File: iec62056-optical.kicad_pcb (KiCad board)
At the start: 2 copper layers, 30 x 30 mm, 5 parts, among them J1 Conn_01x04_Male, Q1 Q_Photo_NPN

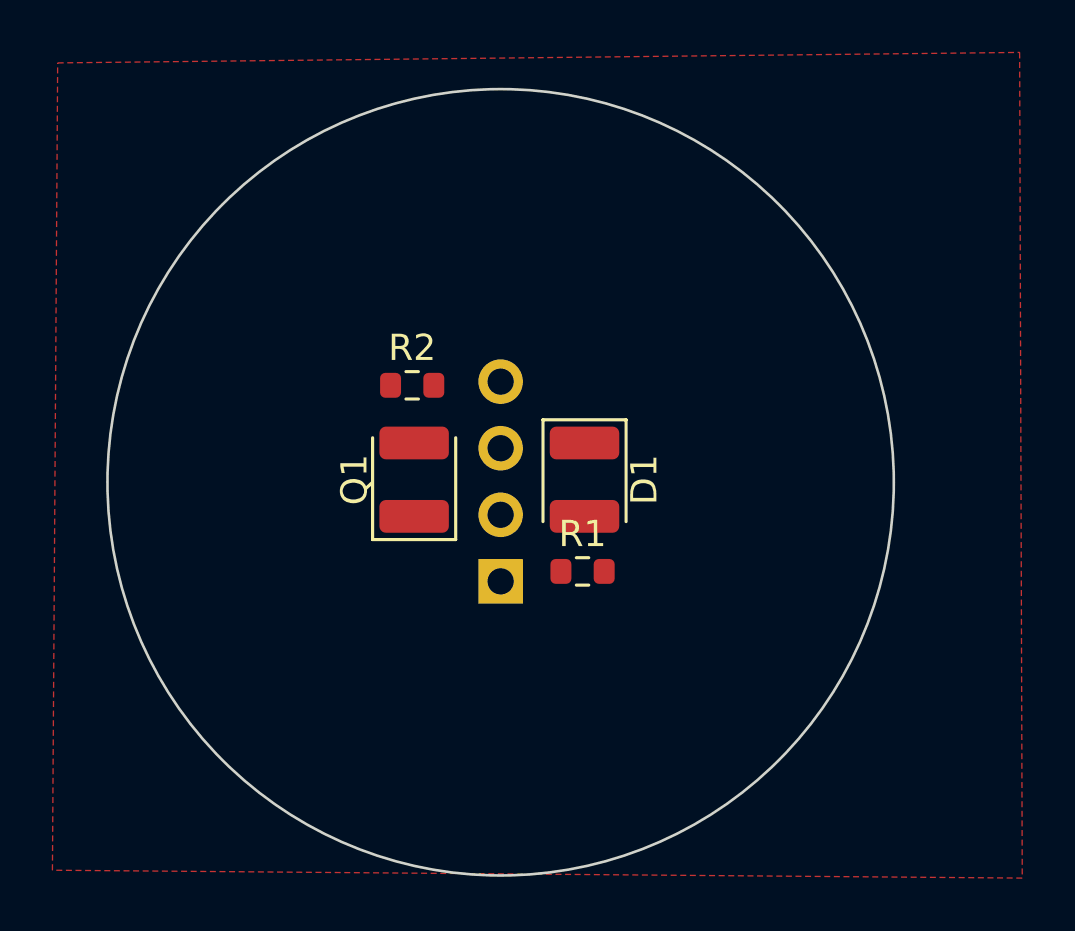
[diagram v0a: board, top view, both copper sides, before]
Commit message: version 1.0
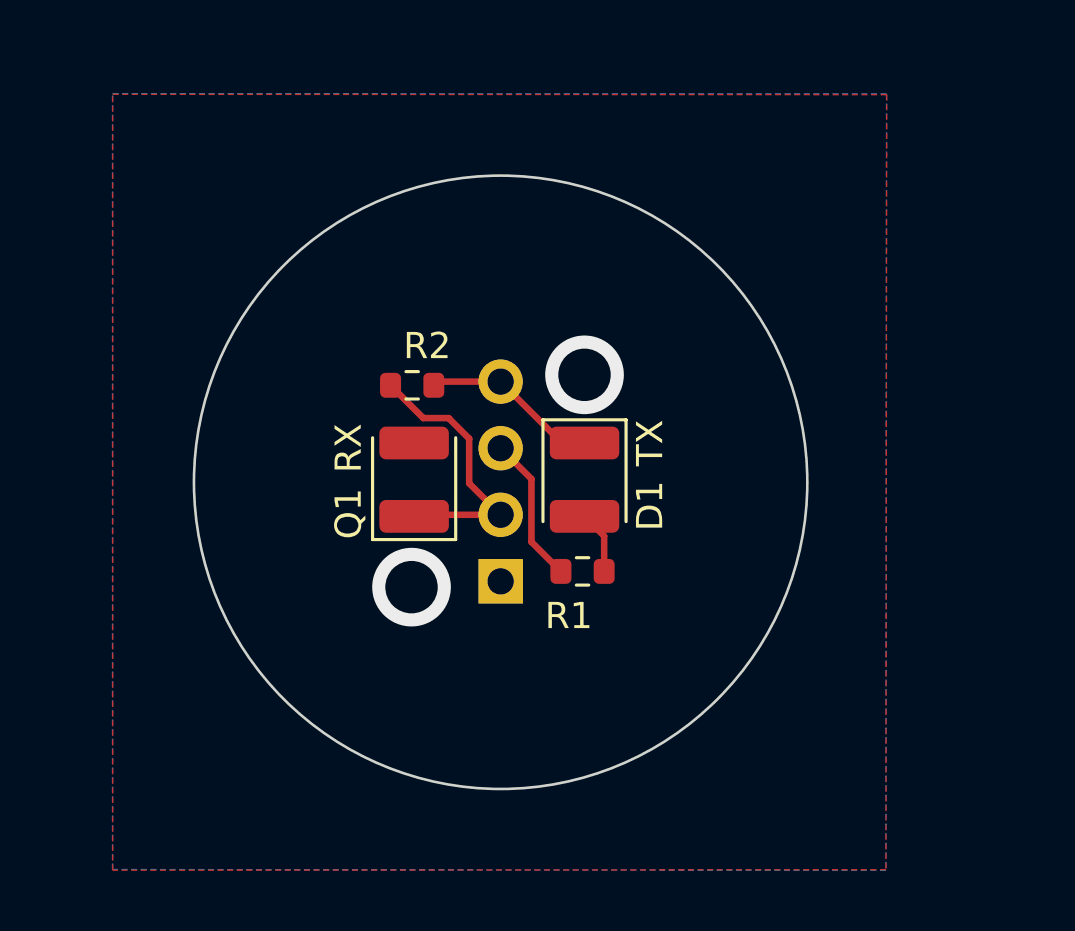
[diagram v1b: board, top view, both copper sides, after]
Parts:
- D1: value LED -> IR42-21C
- Q1: value Q_Photo_NPN -> PT42-21B
- R1: value R -> 0R
- R2: value R -> 1k8
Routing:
- net RXD: track 0.00 -> 10.6 mm
- net +3V3: track 0.00 -> 6.78 mm
- net TXD: track 0.00 -> 5.65 mm
- net Net-(D1-Pad2): track 0.00 -> 2.41 mm
- net GND: vias 0 -> 2
- added copper zone on B.Cu, net GND
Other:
- board size 30 x 30 mm -> 23.4 x 23.4 mm
- board text added: "3V3"
- board text added: "RX"
- board text added: "RXD-PD"
- board text added: "TX"
- board text added: "TXD-LED"
- board text added: "iec62056-optical v1.0 danman.eu"
- board text removed: "RXD"
- board text removed: "TXD"
- board text removed: "VCC"
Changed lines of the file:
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@@
       (outputformat 1)
       (mirror false)
-      (drillshape 1)
+      (drillshape 0)
       (scaleselection 1)
-      (outputdirectory "")
+      (outputdirectory "gerber/")
     )
   )
@@
     (descr "Resistor SMD 0603 (1608 Metric), square (rectangular) end terminal, IPC_7351 nominal, (Body size source: IPC-SM-782 page 72, https://www.pcb-3d.com/wordpress/wp-content/uploads/ipc-sm-782a_amendment_1_and_2.pdf), generated with kicad-footprint-generator")
     (tags "resistor")
-    (property "Sheetfile" "iec62056-optical.kicad_sch")
-    (property "Sheetname" "")
-    (attr smd)
-    (fp_text reference "R2" (at 0 -1.43) (layer "F.SilkS")
-      (effects (font (size 1 1) (thickness 0.15)))
-    )
-    (fp_text value "R" (at 0 1.43) (layer "F.Fab")
+    (property "LCSC" "C185354")
+    (property "Sheetfile" "iec62056-optical.kicad_sch")
+    (property "Sheetname" "")
+    (attr smd)
+    (fp_text reference "R2" (at 0.575 -1.5) (layer "F.SilkS")
+      (effects (font (size 1 1) (thickness 0.15)))
+    )
+    (fp_text value "1k8" (at 0 1.43) (layer "F.Fab")
       (effects (font (size 1 1) (thickness 0.15)))
     )
@@
     (descr "LED SMD 1210 (3225 Metric), square (rectangular) end terminal, IPC_7351 nominal, (Body size source: http://www.tortai-tech.com/upload/download/2011102023233369053.pdf), generated with kicad-footprint-generator")
     (tags "LED")
-    (property "Sheetfile" "iec62056-optical.kicad_sch")
-    (property "Sheetname" "")
-    (attr smd)
-    (fp_text reference "D1" (at 0 -2.28 90) (layer "F.SilkS")
-      (effects (font (size 1 1) (thickness 0.15)))
-    )
-    (fp_text value "LED" (at 0 2.28 90) (layer "F.Fab")
+    (property "LCSC" "C131198")
+    (property "Sheetfile" "iec62056-optical.kicad_sch")
+    (property "Sheetname" "")
+    (attr smd)
+    (fp_text reference "D1" (at 1 -2.5 90) (layer "F.SilkS")
+      (effects (font (size 1 1) (thickness 0.15)))
+    )
+    (fp_text value "IR42-21C" (at 0 2.28 90) (layer "F.Fab")
       (effects (font (size 1 1) (thickness 0.15)))
     )
@@
     (descr "Resistor SMD 0603 (1608 Metric), square (rectangular) end terminal, IPC_7351 nominal, (Body size source: IPC-SM-782 page 72, https://www.pcb-3d.com/wordpress/wp-content/uploads/ipc-sm-782a_amendment_1_and_2.pdf), generated with kicad-footprint-generator")
     (tags "resistor")
-    (property "Sheetfile" "iec62056-optical.kicad_sch")
-    (property "Sheetname" "")
-    (attr smd)
-    (fp_text reference "R1" (at 0 -1.43) (layer "F.SilkS")
-      (effects (font (size 1 1) (thickness 0.15)))
-    )
-    (fp_text value "R" (at 0 1.43) (layer "F.Fab")
+    (property "LCSC" "C95177")
+    (property "Sheetfile" "iec62056-optical.kicad_sch")
+    (property "Sheetname" "")
+    (attr smd)
+    (fp_text reference "R1" (at -0.525 1.7) (layer "F.SilkS")
+      (effects (font (size 1 1) (thickness 0.15)))
+    )
+    (fp_text value "0R" (at 0 1.43) (layer "F.Fab")
       (effects (font (size 1 1) (thickness 0.15)))
     )
@@
     (descr "LED SMD 1210 (3225 Metric), square (rectangular) end terminal, IPC_7351 nominal, (Body size source: http://www.tortai-tech.com/upload/download/2011102023233369053.pdf), generated with kicad-footprint-generator")
     (tags "LED")
-    (property "Sheetfile" "iec62056-optical.kicad_sch")
-    (property "Sheetname" "")
-    (attr smd)
-    (fp_text reference "Q1" (at 0 -2.28 90) (layer "F.SilkS")
-      (effects (font (size 1 1) (thickness 0.15)))
-    )
-    (fp_text value "Q_Photo_NPN" (at 0 2.28 90) (layer "F.Fab")
+    (property "LCSC" "C131199")
+    (property "Sheetfile" "iec62056-optical.kicad_sch")
+    (property "Sheetname" "")
+    (attr smd)
+    (fp_text reference "Q1" (at -1.3 -2.5 90) (layer "F.SilkS")
+      (effects (font (size 1 1) (thickness 0.15)))
+    )
+    (fp_text value "PT42-21B" (at 0 2.28 90) (layer "F.Fab")
       (effects (font (size 1 1) (thickness 0.15)))
     )
@@
     (property "Sheetname" "")
     (attr through_hole)
-    (fp_text reference "J1" (at 0 2.33) (layer "B.SilkS")
+    (fp_text reference "J1" (at 2.6 -3.68) (layer "B.SilkS")
       (effects (font (size 1 1) (thickness 0.15)) (justify mirror))
     )
@@
   )
   (gr_circle (center 155.9 92) (end 166.745275 92) (layer "F.Mask") (width 8) (fill none))
-  (gr_circle (center 155.9 92) (end 170.9 92) (layer "Edge.Cuts") (width 0.1) (fill none))
-  (gr_text "RXD" (at 147.5 89.3) (layer "B.SilkS")
-    (effects (font (size 1 1) (thickness 0.15)) (justify mirror))
-  )
-  (gr_text "VCC" (at 144.6 91.8) (layer "B.SilkS")
-    (effects (font (size 1 1) (thickness 0.15)) (justify mirror))
-  )
-  (gr_text "GND" (at 147.6 94.2) (layer "B.SilkS")
-    (effects (font (size 1 1) (thickness 0.15)) (justify mirror))
-  )
-  (gr_text "TXD" (at 147.5 87.5) (layer "B.SilkS")
+  (gr_circle (center 155.9 92) (end 167.6 92) (layer "Edge.Cuts") (width 0.1) (fill none))
+  (gr_text "RXD-PD" (at 151.1 93.3) (layer "B.SilkS")
+    (effects (font (size 1 1) (thickness 0.15)) (justify mirror))
+  )
+  (gr_text "3V3" (at 152.7 88) (layer "B.SilkS")
+    (effects (font (size 1 1) (thickness 0.15)) (justify mirror))
+  )
+  (gr_text "GND" (at 159 95.9) (layer "B.SilkS")
+    (effects (font (size 1 1) (thickness 0.15)) (justify mirror))
+  )
+  (gr_text "TXD-LED" (at 150.7 90.8) (layer "B.SilkS")
+    (effects (font (size 1 1) (thickness 0.15)) (justify mirror))
+  )
+  (gr_text "iec62056-optical v1.0\ndanman.eu" (at 156 99.8) (layer "B.SilkS")
     (effects (font (size 1 1) (thickness 0.15)) (justify mirror))
   )
@@
     (effects (font (size 1 1) (thickness 0.15)) (justify mirror))
   )
-  (dimension (type aligned) (layer "Edge.Cuts")
+  (gr_text "TX" (at 161.6 90.5 90) (layer "F.SilkS")
+    (effects (font (size 1 1) (thickness 0.15)))
+  )
+  (gr_text "RX" (at 150.1 90.7 90) (layer "F.SilkS")
+    (effects (font (size 1 1) (thickness 0.15)))
+  )
+  (dimension (type aligned) (layer "Cmts.User")
     (pts (xy 152.6 91.4) (xy 159.1 91.4))
     (height 7.6)
-    (gr_text "6,5000 mm" (at 155.85 97.85) (layer "Edge.Cuts")
+    (gr_text "6,5000 mm" (at 155.85 97.85) (layer "Cmts.User")
       (effects (font (size 1 1) (thickness 0.15)))
     )
@@
     (style (thickness 0.1) (arrow_length 1.27) (text_position_mode 0) (extension_height 0.58642) (extension_offset 0.5) keep_text_aligned)
   )
+  (segment (start 158.24 90.5) (end 155.9 88.16) (width 0.25) (layer "F.Cu") (net 1))
+  (segment (start 153.49 88.16) (end 153.35 88.3) (width 0.25) (layer "F.Cu") (net 1))
+  (segment (start 159.1 90.5) (end 158.24 90.5) (width 0.25) (layer "F.Cu") (net 1))
+  (segment (start 155.9 88.16) (end 153.49 88.16) (width 0.25) (layer "F.Cu") (net 1))
+  (segment (start 159.85 94.05) (end 159.1 93.3) (width 0.25) (layer "F.Cu") (net 2))
+  (segment (start 159.85 95.4) (end 159.85 94.05) (width 0.25) (layer "F.Cu") (net 2))
+  (segment (start 154.7 92.04) (end 155.9 93.24) (width 0.25) (layer "F.Cu") (net 3))
+  (segment (start 152.95048 89.55048) (end 153.912973 89.55048) (width 0.25) (layer "F.Cu") (net 3))
+  (segment (start 154.7 90.337507) (end 154.7 92.04) (width 0.25) (layer "F.Cu") (net 3))
+  (segment (start 152.6 93.3) (end 152.66 93.24) (width 0.25) (layer "F.Cu") (net 3))
+  (segment (start 151.7 88.3) (end 152.95048 89.55048) (width 0.25) (layer "F.Cu") (net 3))
+  (segment (start 152.66 93.24) (end 155.9 93.24) (width 0.25) (layer "F.Cu") (net 3))
+  (segment (start 153.912973 89.55048) (end 154.7 90.337507) (width 0.25) (layer "F.Cu") (net 3))
+  (segment (start 157.074511 91.874511) (end 157.074511 94.274511) (width 0.25) (layer "F.Cu") (net 4))
+  (segment (start 155.9 90.7) (end 157.074511 91.874511) (width 0.25) (layer "F.Cu") (net 4))
+  (segment (start 157.074511 94.274511) (end 158.2 95.4) (width 0.25) (layer "F.Cu") (net 4))
+  (via (at 152.5 96) (size 3) (drill 2) (layers "F.Cu" "B.Cu") (free) (net 5))
+  (via (at 159.1 87.9) (size 3) (drill 2) (layers "F.Cu" "B.Cu") (free) (net 5))
   (zone (net 5) (net_name "GND") (layer "F.Cu") (hatch edge 0.508)
     (connect_pads (clearance 0.508))
@@
     (polygon
       (pts
-        (xy 175.8 107.1)
-        (xy 138.8 106.8)
-        (xy 139 76)
-        (xy 175.7 75.6)
+        (xy 170.6 106.77935)
+        (xy 141.099726 106.800866)
+        (xy 141.099491 77.199324)
+        (xy 170.628427 77.213225)
       )
     )
+  )
+  (zone (net 5) (net_name "GND") (layer "B.Cu") (hatch edge 0.508)
+    (connect_pads (clearance 0.508))
+    (min_thickness 0.254) (filled_areas_thickness no)
+    (fill yes (thermal_gap 0.508) (thermal_bridge_width 0.508))
+    (polygon
+      (pts
+        (xy 170.6 106.8)
+        (xy 141.093462 106.773204)
+        (xy 141.093227 77.171662)
+        (xy 170.622163 77.185563)
+      )
+    )
